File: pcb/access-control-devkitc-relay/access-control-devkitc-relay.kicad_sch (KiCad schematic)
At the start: 15 parts, among them K1 G5LE-1

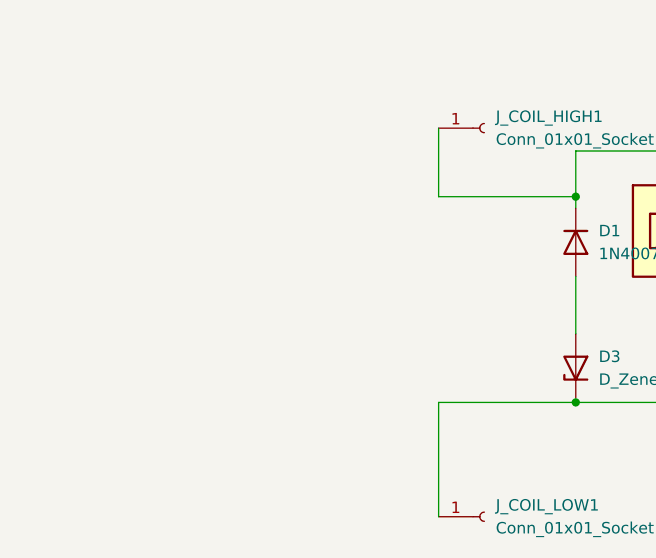
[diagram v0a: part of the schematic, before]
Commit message: Final changes pre manufacture
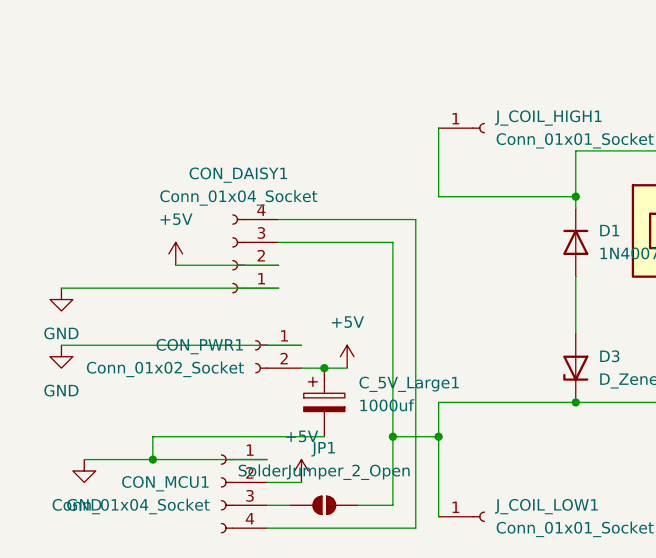
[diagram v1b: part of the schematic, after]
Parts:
- added CON_DAISY1: Conn_01x04_Socket, Connector_JST:JST_XA_B04B-XASK-1_1x04_P2.50mm_Vertical, symbol Connector:Conn_01x04_Socket
- added CON_MCU1: Conn_01x04_Socket, Connector_PinHeader_2.54mm:PinHeader_1x04_P2.54mm_Vertical, symbol Connector:Conn_01x04_Socket
- added CON_PWR1: Conn_01x02_Socket, Connector_JST:JST_XH_B2B-XH-A_1x02_P2.50mm_Vertical, symbol Connector:Conn_01x02_Socket
- added C_5V_Large1: 1000uf, Capacitor_THT:CP_Radial_D8.0mm_P5.00mm, symbol Device:C_Polarized
- added JP1: SolderJumper_2_Open, Jumper:SolderJumper-2_P1.3mm_Open_TrianglePad1.0x1.5mm, symbol Jumper:SolderJumper_2_Open
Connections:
- net +5V: now also CON_DAISY1.2 (Pin_2), CON_MCU1.2 (Pin_2), CON_PWR1.2 (Pin_2), C_5V_Large1.1
- net at D3.1 (K), J_COIL_LOW1.1 (Pin_1), K1.2: now also CON_DAISY1.3 (Pin_3), JP1.2 (B)
- new net: CON_MCU1.3 (Pin_3), JP1.1 (A)
- new net: CON_DAISY1.4 (Pin_4), CON_MCU1.4 (Pin_4)
- new net GND: CON_DAISY1.1 (Pin_1), CON_MCU1.1 (Pin_1), CON_PWR1.1 (Pin_1), C_5V_Large1.2
